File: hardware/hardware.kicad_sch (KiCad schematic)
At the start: 102 parts, among them IC1 TAS5760LDAPR, J1 GMC020080HR, J2 Conn_01x04, J3 Conn_01x04, J4 USB-C, SW1 SW_Push, SW2 SW_Push, SW3 SW_Push, SW5 SW_Push, U1 TPS563200, U2 ESP32-S3, U3 USBLC6-2SC6, Y1 40MHz, Y2 ABS07-166-32.768KHZ-T

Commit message: usb
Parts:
- U3: footprint Package_TO_SOT_SMD:TSOT-23-6_HandSoldering -> SamacSys_Parts:SOT95P280X145-6N
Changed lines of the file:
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@@
 			)
 		)
-		(property "Footprint" "Package_TO_SOT_SMD:TSOT-23-6_HandSoldering"
+		(property "Footprint" "SamacSys_Parts:SOT95P280X145-6N"
 			(at 293.37 134.62 0)
 			(effects

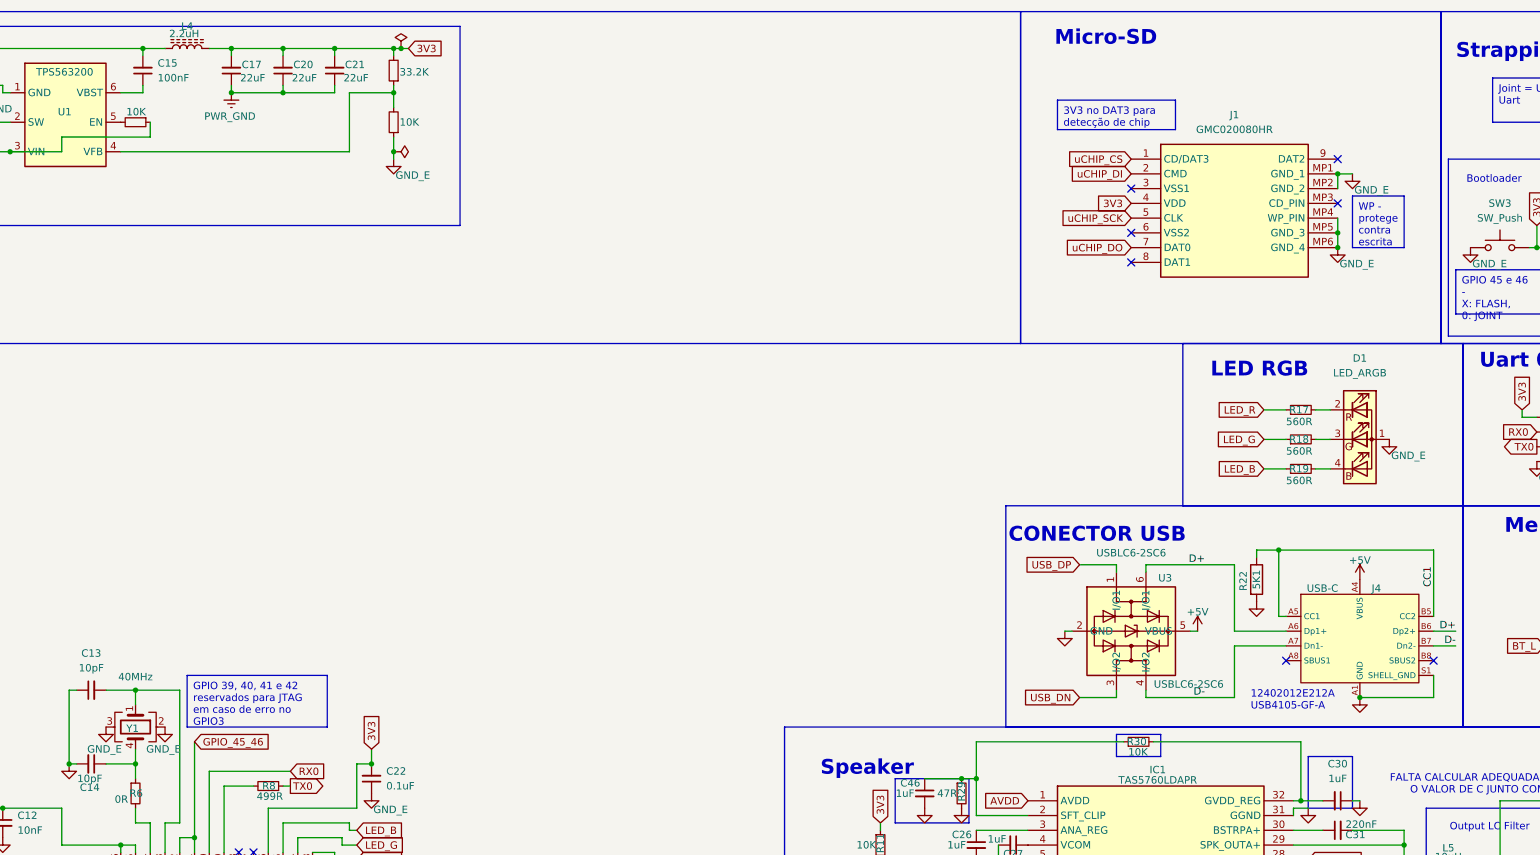
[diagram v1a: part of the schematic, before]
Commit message: desacoplamento
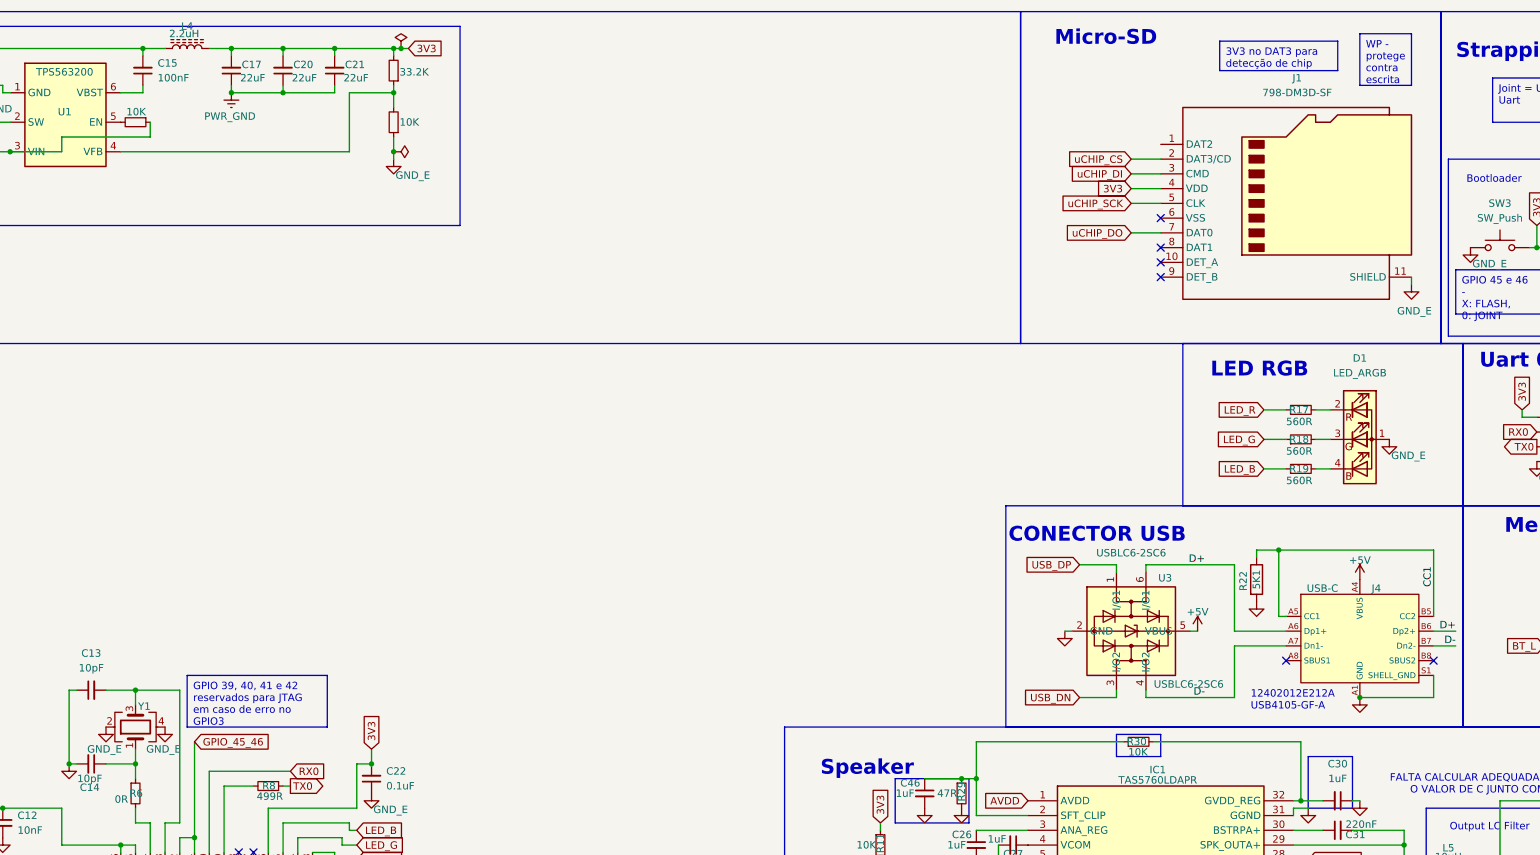
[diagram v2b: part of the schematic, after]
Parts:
- removed Y1: 40MHz, Crystal:Crystal_SMD_2520-4Pin_2.5x2.0mm, symbol Device:Crystal_GND23
- added Y1: ECS-400-10-36B2-CKM-TR, Crystal:Crystal_SMD_2520-4Pin_2.5x2.0mm, symbol Device:Crystal_GND24
- J1: value GMC020080HR -> 798-DM3D-SF; symbol GMC020080HR:GMC020080HR -> Connector:Micro_SD_Card_Det_Hirose_DM3AT
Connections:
- net 3V3: now also J1.2 (DAT3/CD); no longer J1.1 (CD/DAT3)
- net GND_E: now also J1.11 (SHIELD), Y1.2, Y1.4; no longer J1.MP1 (GND_1), J1.MP2 (GND_2), J1.MP4 (WP_PIN), J1.MP5 (GND_3), J1.MP6 (GND_4)
- net uCHIP_DI: now also J1.3 (CMD); no longer J1.2 (CMD)
- net at C13.2, U2.53 (XTAL_N): now also Y1.3
- net at C14.1, R6.1: now also Y1.1
- no-connect marks 23 -> 22
